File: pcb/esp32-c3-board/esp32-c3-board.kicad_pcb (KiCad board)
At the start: 2 copper layers, 118.7 x 40.6 mm, 30 parts, among them P101 CAN, P102 BMS UART, P3 CONN_1, P4 CONN_1, P5 CONN_1, P6 CONN_1, U102 TJA1050, U2 esp32-c3-ebay, U4 6N137, U5 DCDCConverter, U6 6N137

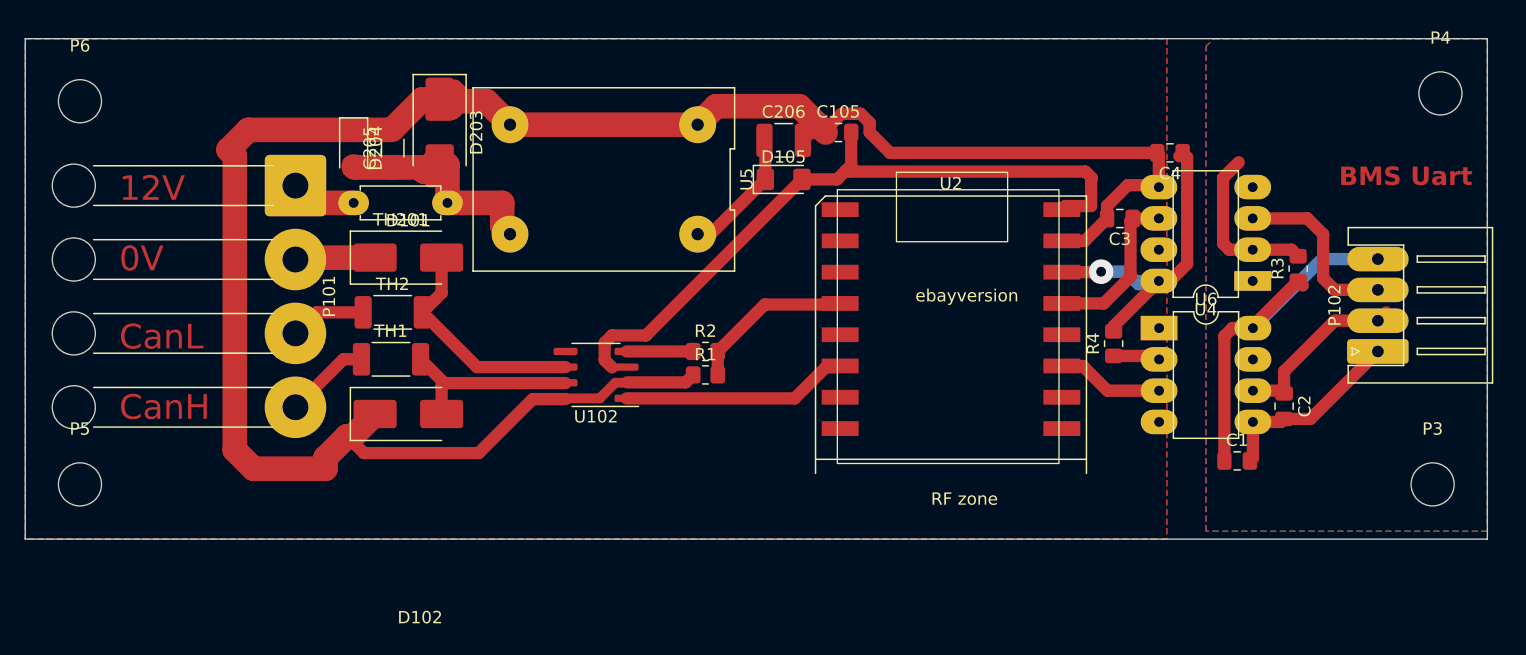
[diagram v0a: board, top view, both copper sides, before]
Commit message: Working version connected to real BMS
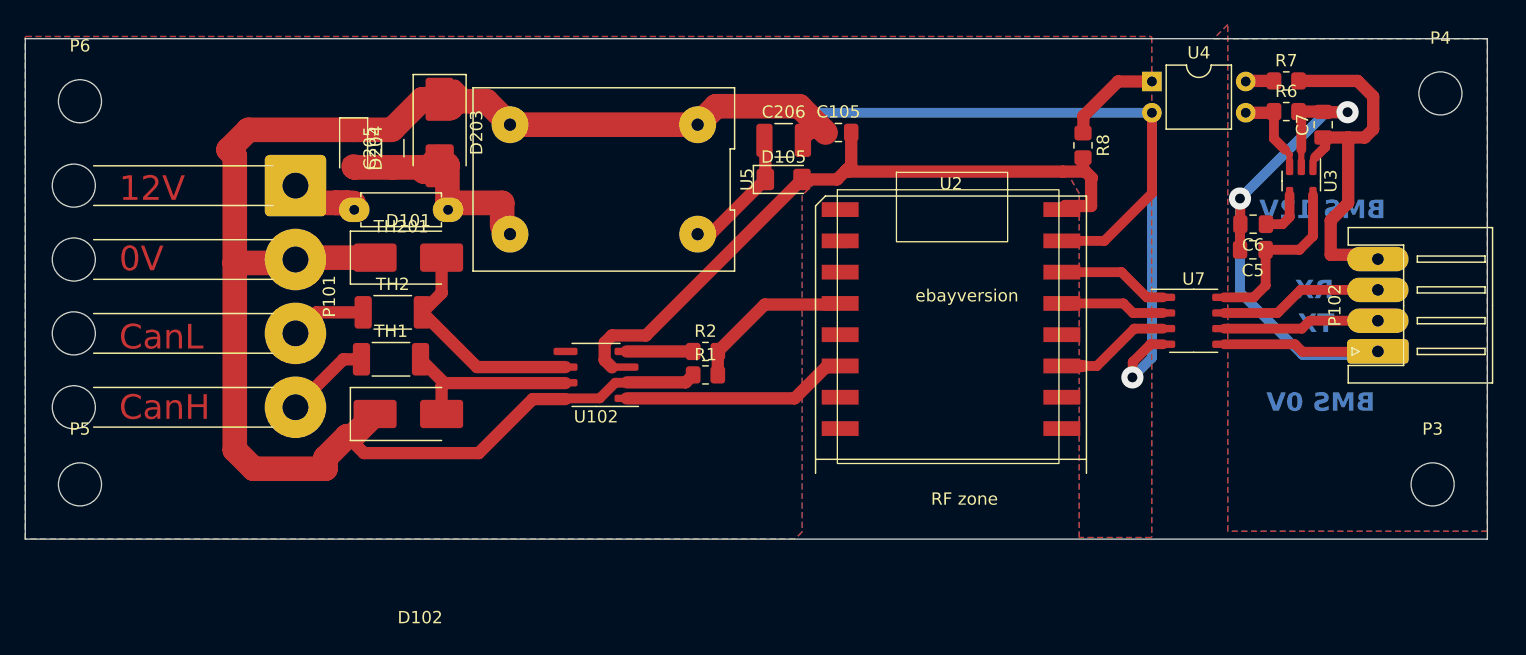
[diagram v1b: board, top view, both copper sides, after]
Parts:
- removed C1, C4: 100nF, Capacitor_SMD:C_0805_2012Metric_Pad1.18x1.45mm_HandSolder
- removed C2, C3: 15pF, Capacitor_SMD:C_0805_2012Metric_Pad1.18x1.45mm_HandSolder
- removed R3: 2K2, Resistor_SMD:R_0805_2012Metric_Pad1.20x1.40mm_HandSolder
- removed R4: 1K, Resistor_SMD:R_0805_2012Metric_Pad1.20x1.40mm_HandSolder
- removed U6: 6N137, Package_DIP:DIP-8_W7.62mm
- added C5: 10uF, Capacitor_SMD:C_0805_2012Metric_Pad1.18x1.45mm_HandSolder, F.Cu at (112.4, 57.1)
- added C6: 10nF, Capacitor_SMD:C_0805_2012Metric_Pad1.18x1.45mm_HandSolder, F.Cu at (112.4, 55.1)
- added C7: 10uF, Capacitor_SMD:C_0805_2012Metric_Pad1.18x1.45mm_HandSolder, F.Cu at (118.1, 47.0)
- added R6: 3K3, Resistor_SMD:R_0805_2012Metric_Pad1.20x1.40mm_HandSolder, F.Cu at (115.1, 45.9)
- added R7: 10K, Resistor_SMD:R_0805_2012Metric_Pad1.20x1.40mm_HandSolder, F.Cu at (115.1, 43.4)
- added R8: 10K, Resistor_SMD:R_0805_2012Metric_Pad1.20x1.40mm_HandSolder, F.Cu at (98.6, 48.7)
- added U3: LP2985-3.3, Package_TO_SOT_SMD:SOT-23-5, F.Cu at (116.3, 51.6)
- added U7: STIS0621, Package_SO:SOIC-8_3.9x4.9mm_P1.27mm, F.Cu at (107.6, 62.9)
- U4: value 6N137 -> PC817; footprint Package_DIP:DIP-8_W7.62mm -> Package_DIP:DIP-4_W7.62mm
- moved U4 18.2 mm to (104.2, 43.5), turned to 0 degrees
- moved TH201 0.56 mm to (47.0, 53.9)
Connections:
- net Net-(D203-K) renamed 12vFused
- P102 pad 4: 5V BMS -> 12V BMS
- U4 pad 1: unconnected-(U4-NC-Pad1) -> Net-(R8-Pad1)
- U4 pad 2: Net-(U4-A) -> GND
- U4 pad 3: RX from BMS -> Net-(U3-ON/~{OFF})
- U4 pad 4: (no net) -> Net-(R7-Pad1)
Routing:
- net GND BMS: track 15.8 -> 58.3 mm, vias 0 -> 2
- net GND: track 176.3 -> 218.2 mm, vias 0 -> 1
- net 12V BMS: track 0.00 -> 31.2 mm
- net 5V BMS: track 31.1 -> 0.00 mm
- net 3v3: track 26.8 -> 9.08 mm, vias 1 -> 0
- net 3.3V BMS: track 0.00 -> 14.3 mm
- net Net-(U4-A): track 13.7 -> 0.00 mm
- net Net-(R8-Pad1): track 0.00 -> 8.12 mm
- net Net-(U3-ON/~{OFF}): track 0.00 -> 7.36 mm
- net BMS-RX: track 14.3 -> 9.46 mm
- net Net-(U3-BP): track 0.00 -> 3.96 mm
- net Net-(U6-A): track 3.81 -> 0.00 mm
- net Net-(R7-Pad1): track 0.00 -> 2.31 mm
- net TX to BMS: track 14.7 -> 12.8 mm
- net 12v: track 5.31 -> 7.06 mm
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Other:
- board text added: "BMS 0V"
- board text added: "BMS 12V"
- board text added: "RX"
- board text added: "TX"
- board text removed: "BMS Uart"
